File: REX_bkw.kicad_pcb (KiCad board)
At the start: 2 copper layers, 16 x 38 mm, 11 parts, among them J1 Molex_DIP28_edge_contacts, J2 JTAG, J3 PRG, U1 XCR3064XL-10VQ44, U2 29F800, U3 LP2980

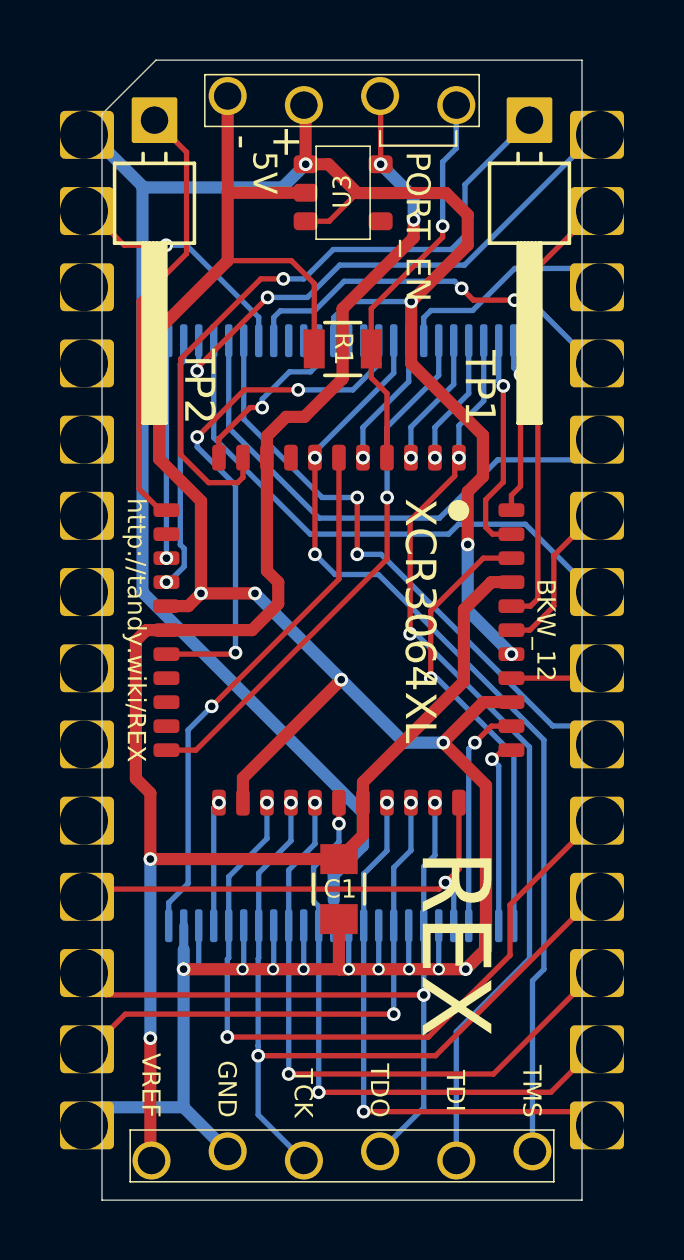
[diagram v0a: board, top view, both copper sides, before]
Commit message: v13
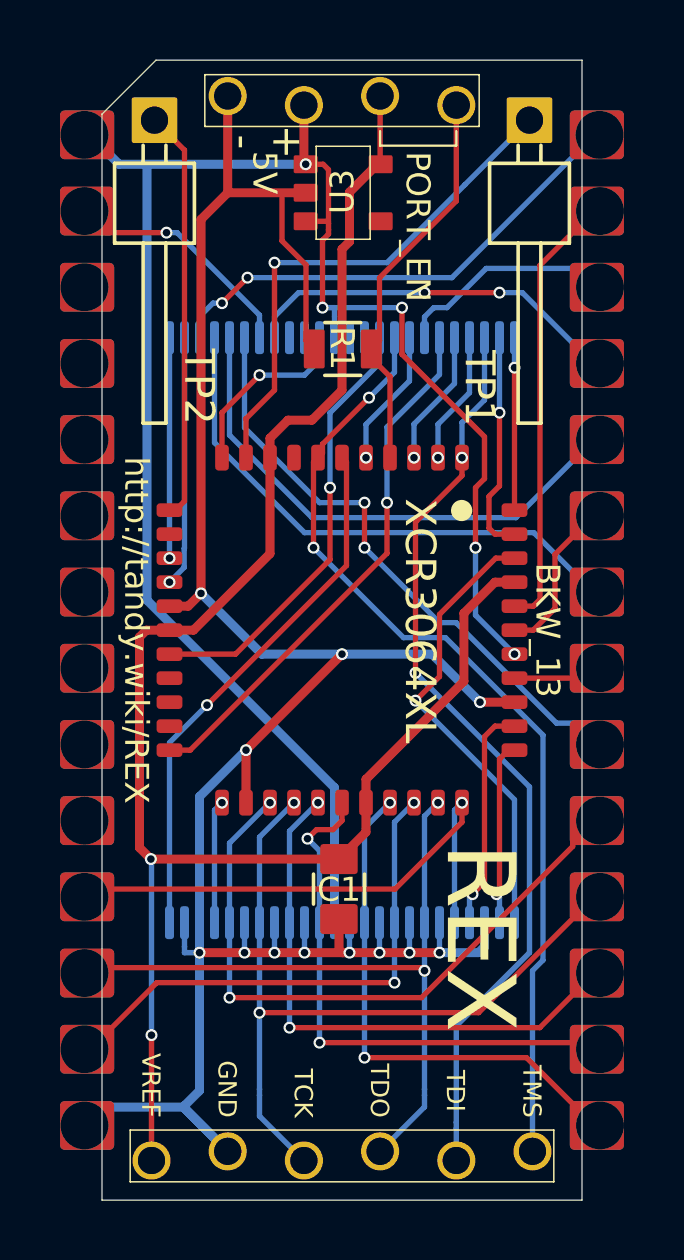
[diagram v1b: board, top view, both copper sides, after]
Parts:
- added NT1: Net-Tie_2, 000_LOCAL:Net_Tie_2_0.18mm, F.Cu at (146.8, 85.7)
- added NT2: Net-Tie_2, 000_LOCAL:Net_Tie_2_0.18mm, B.Cu at (142.0, 109.8)
- added NT3: Net-Tie_2, 000_LOCAL:Net_Tie_2_0.18mm, B.Cu at (144.5, 114.6)
- added NT4: Net-Tie_2, 000_LOCAL:Net_Tie_2_0.18mm, B.Cu at (150.0, 114.6)
- added NT5: Net-Tie_2, 000_LOCAL:Net_Tie_2_0.18mm, B.Cu at (151.0, 115.7)
- added NT6: Net-Tie_2, 000_LOCAL:Net_Tie_2_0.18mm, B.Cu at (153.6, 114.6)
- C1: footprint Capacitors_SMD:C_0805 -> 000_LOCAL:C_0805
- R1: footprint Resistors_SMD:R_0805 -> 000_LOCAL:R_0805
- moved U2 0.10 mm to (147.2, 99.2)
- moved U1 0.10 mm to (147.2, 99.2)
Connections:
- net /AD0 renamed /D0
- net /AD2 renamed /D2
- net /AD3 renamed /D3
- net /AD4 renamed /D4
- net /AD5 renamed /D5
- net /AD7 renamed /D7
- J1 pad 12: /AD1 -> /D1
- J1 pad 18: /AD6 -> /D6
- J2 pad 3: /AD6 -> /TCK
- J2 pad 4: /AD1 -> /TDO
- J2 pad 5: /LVA4 -> /TDI
- J2 pad 6: /LVA19 -> /TMS
- U1 pad 26: /AD6 -> /D6
- U1 pad 32: /AD1 -> /D1
- U1 pad 38: /+5 -> /~RESET
- U2 pad 12: /+5 -> /~RESET
- U2 pad 31: /AD1 -> /D1
- U2 pad 42: /AD6 -> /D6
- U2 pad 47: GND -> /~BYTE
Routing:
- net /+5: track 67.8 -> 41.0 mm, vias 4 -> 1
- net /AD6: track 26.6 -> 0.00 mm, vias 2 -> 0
- net /AD1: track 24.0 -> 0.00 mm, vias 2 -> 0
- net /D6: track 0.00 -> 23.0 mm, vias 0 -> 2
- net /D1: track 0.00 -> 21.2 mm, vias 0 -> 2
- net /~RESET: track 0.00 -> 19.7 mm, vias 0 -> 4
- net GND: track 91.2 -> 85.2 mm, vias 13 -> 12
- net /TP1: track 22.3 -> 17.4 mm
- net /TCK: track 0.00 -> 2.79 mm
- net /D7: track 24.8 -> 22.0 mm
- net /RY_BY: track 17.5 -> 14.8 mm, vias 3 -> 1
- net /TDO: track 0.00 -> 2.49 mm
- net +3V3: track 61.0 -> 58.8 mm, vias 4 -> 2
- net /D5: track 21.2 -> 19.0 mm
- net /LVA19: track 32.3 -> 30.3 mm
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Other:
- net class Default: clearance 0.1778 -> 0.16; trace_width 0.1778 -> 0.18; via_dia 0.4572 -> 0.4; via_drill 0.254 -> 0.25
- rule trace_clearance: 0.1778 -> 0.16
- rule trace_min: 0.1778 -> 0.16
- rule via_min_drill: 0.254 -> 0.25
- rule via_min_size: 0.381 -> 0.4
- board text added: "BKW_13"
- board text removed: "BKW_12"
